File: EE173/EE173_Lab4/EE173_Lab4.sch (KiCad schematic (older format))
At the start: 25 parts

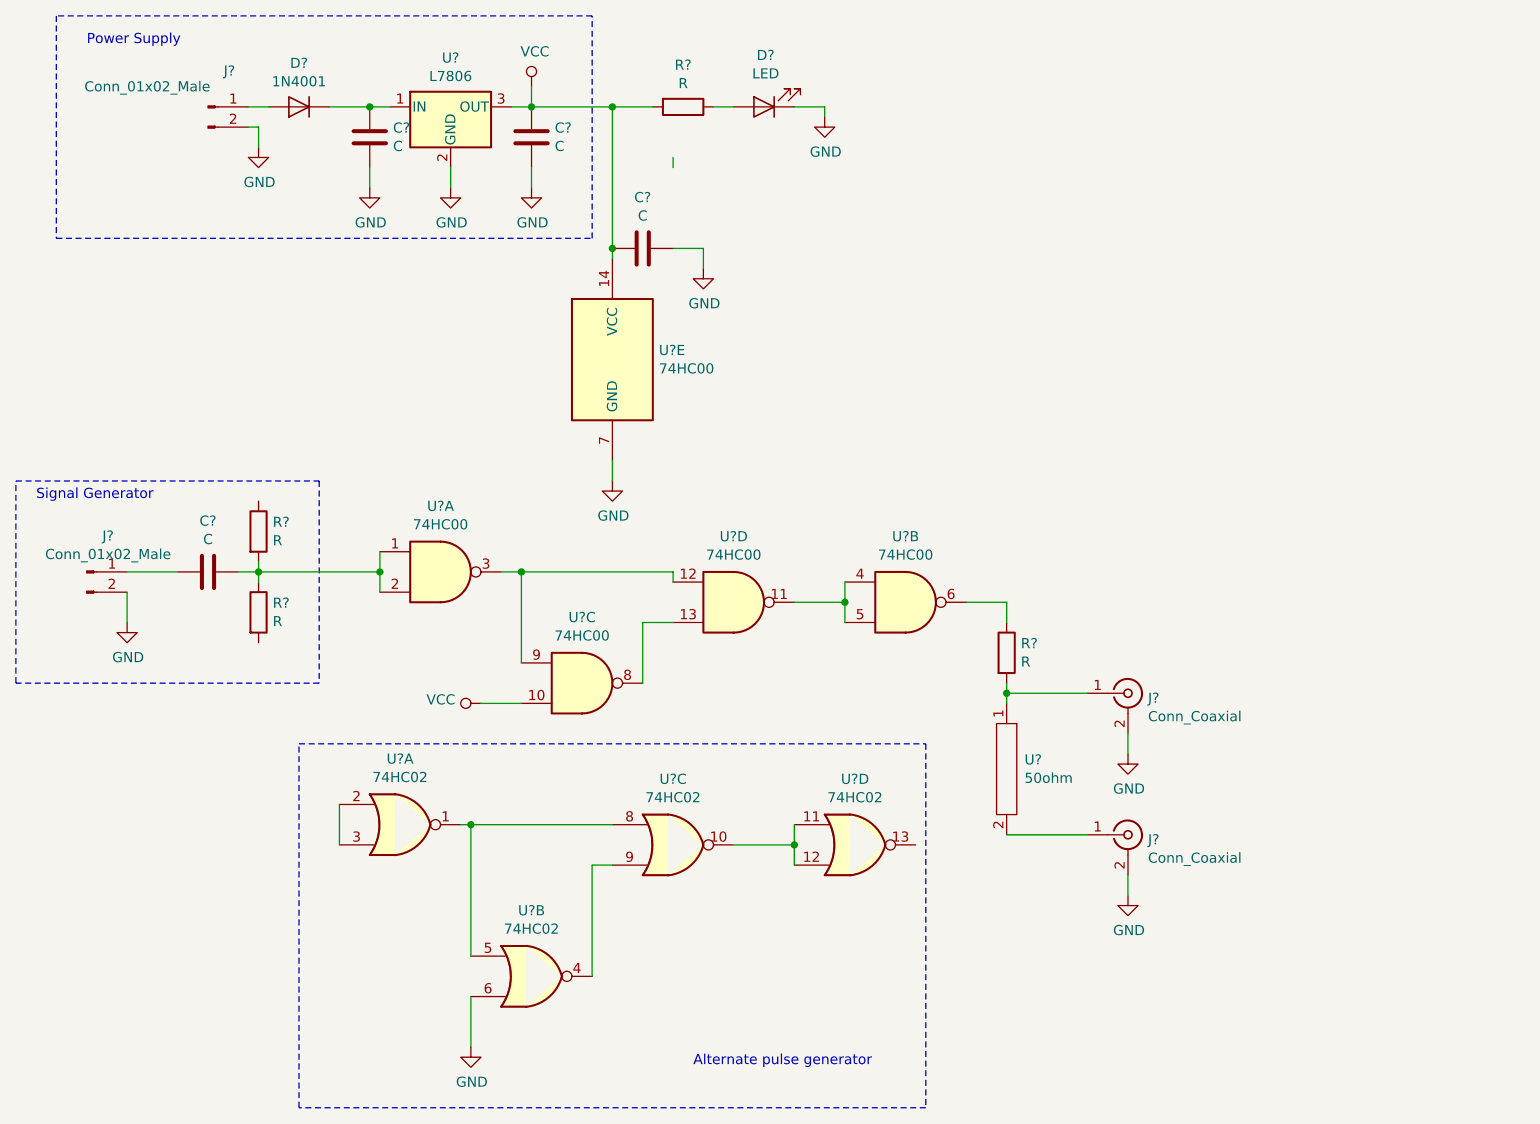
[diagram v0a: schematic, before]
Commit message: Added the jumpers to investigate source reflections. Did not choose values for resistors yet
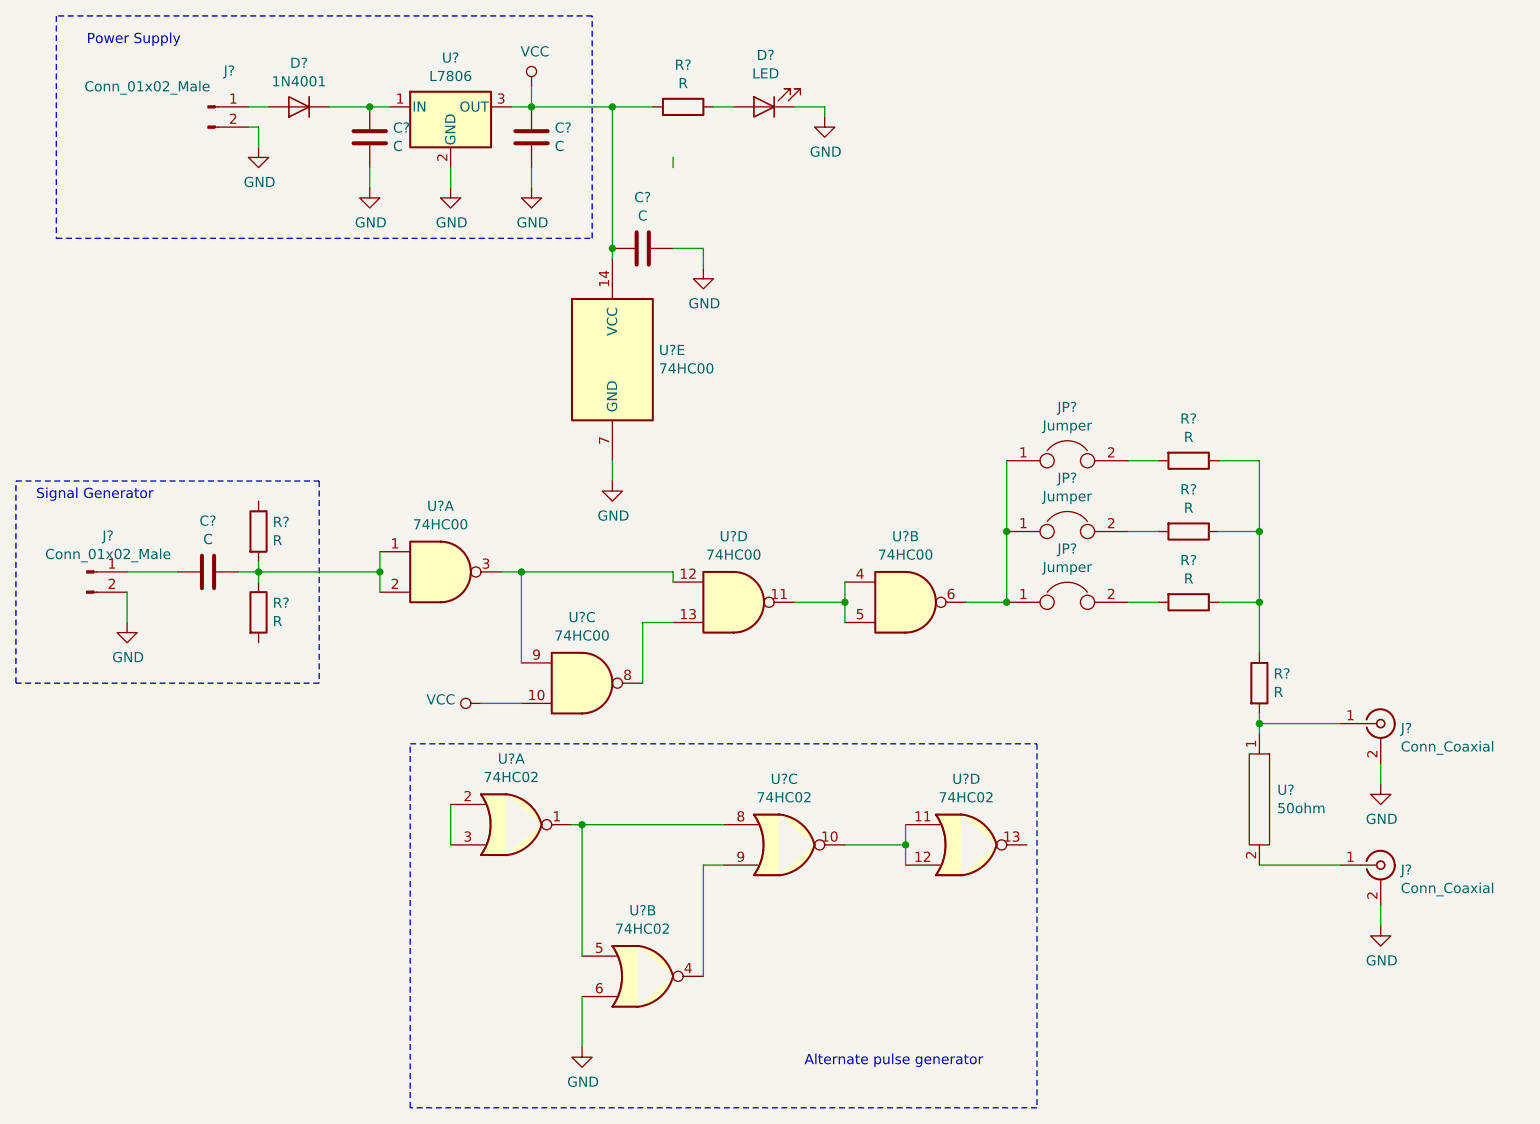
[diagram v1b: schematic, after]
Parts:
- added JP? (x3): Jumper, symbol Device:Jumper
- added R? (x3): R, symbol Device:R
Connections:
- wire segments 57 -> 67
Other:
- moved on the sheet: J?, R?, U?, U?A, U?B, U?C, U?D
